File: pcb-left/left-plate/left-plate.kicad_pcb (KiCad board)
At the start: 2 copper layers, 197.4 x 119.6 mm, 71 parts, among them SW0 SW_PUSH, SW1 SW_PUSH, SW10 SW_PUSH, SW11 SW_PUSH, SW12 SW_PUSH, SW13 SW_PUSH, SW14 SW_PUSH, SW15 SW_PUSH, SW16 SW_PUSH, SW17 SW_PUSH, SW18 SW_PUSH, SW19 SW_PUSH, SW2 SW_PUSH, SW20 SW_PUSH, SW21 SW_PUSH, SW22 SW_PUSH, SW23 SW_PUSH, SW24 SW_PUSH, SW25 SW_PUSH, SW26 SW_PUSH, SW27 SW_PUSH, SW28 SW_PUSH, SW29 SW_PUSH, SW3 SW_PUSH, SW30 SW_PUSH, SW31 SW_PUSH, SW4 SW_PUSH, SW5 SW_PUSH, SW6 SW_PUSH, SW7 SW_PUSH, SW8 SW_PUSH, SW9 SW_PUSH

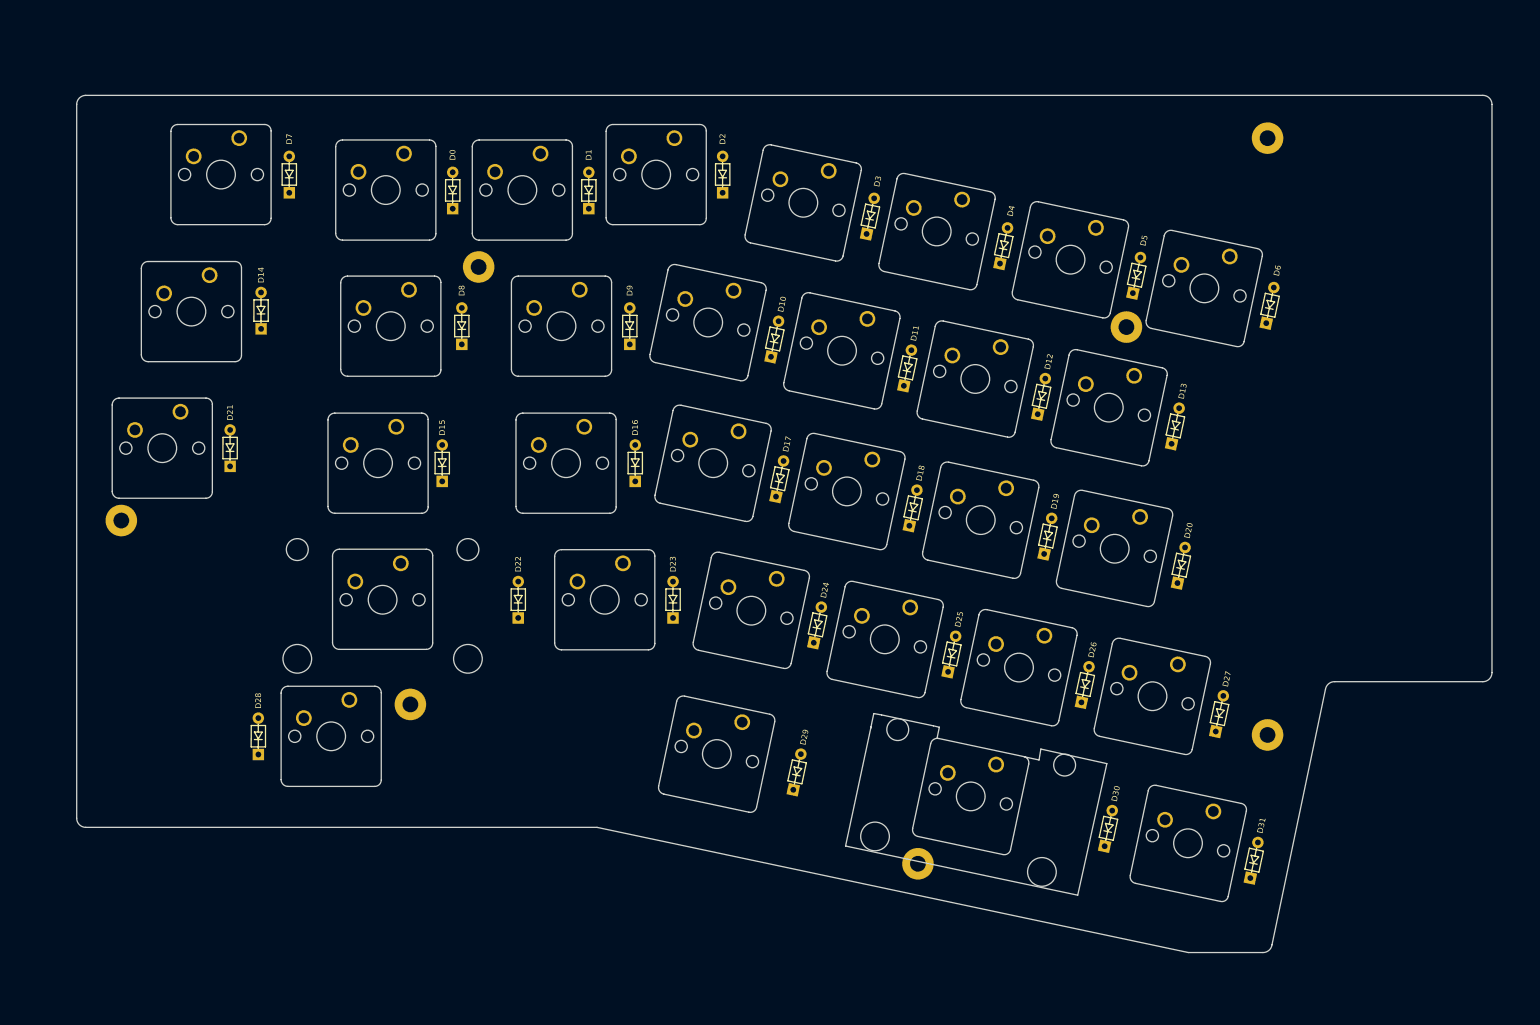
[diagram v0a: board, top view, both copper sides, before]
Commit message: update
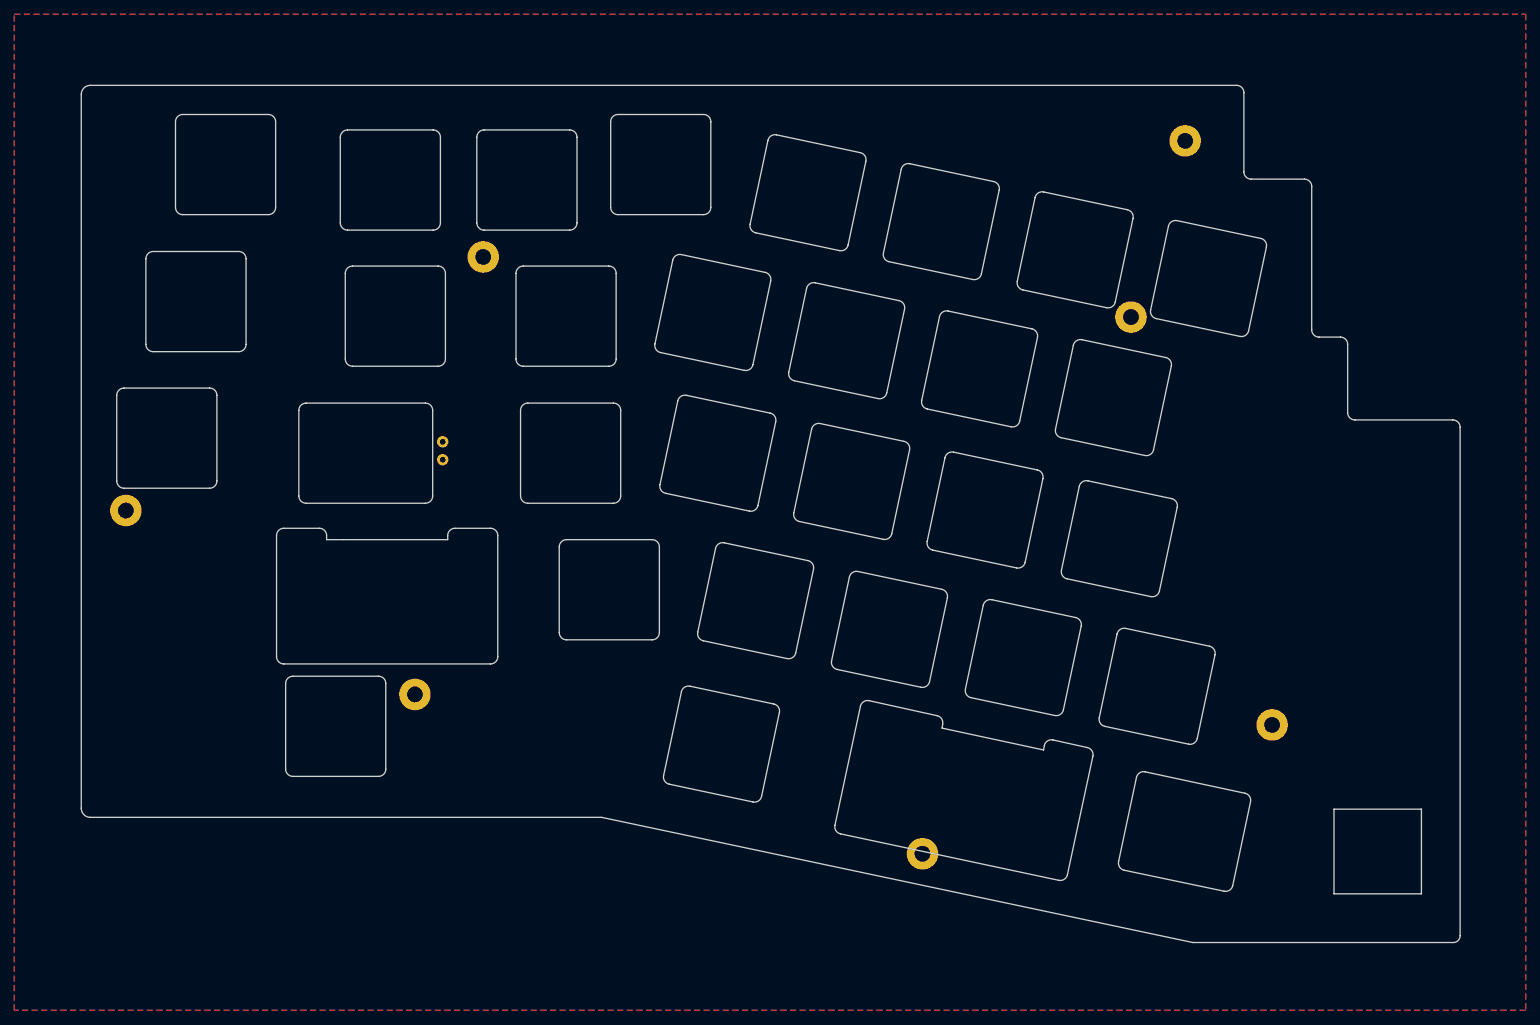
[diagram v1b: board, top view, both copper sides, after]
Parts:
- removed D0, D1, D10, D11, D12, D13, D14, D15, D16, D17, D18, D19, D2, D20, D21, D22, D23, D24, D25, D26, D27, D28, D29, D3, D30, D31, D4, D5, D6, D7, D8, D9: D, cftkb:D_DO-35_SOD27_P5.08mm_Horizontal
- removed SW0, SW1, SW10, SW11, SW12, SW13, SW14, SW16, SW17, SW18, SW19, SW2, SW20, SW21, SW23, SW24, SW25, SW26, SW27, SW3, SW31, SW4, SW5, SW6, SW7, SW9: SW_PUSH, cftkb:SW_Cherry_MX1A_1.00u_PCB-NOSCREEN
- removed SW15: SW_PUSH, cftkb:SW_Cherry_MX1A_1.75u_PCBNOSCREEN
- removed SW22, SW30: SW_PUSH, cftkb:SW_Cherry_MX1A_2.25u_PCBNOSCREEN
- removed SW28, SW29, SW8: SW_PUSH, cftkb:SW_Cherry_MX1A_1.50u_PCBNOSCREEN
- added C1: Device_C_Small, cftkb:C_Disc_D3.0mm_W1.6mm_P2.50mm, B.Cu at (99.5, 84.3)
- moved TH1 11.5 mm to (203.1, 42.3)
- moved TH6 1.53 mm to (195.5, 66.9)
- moved TH2 1.53 mm to (55.3, 93.9)
- moved TH4 1.53 mm to (95.6, 119.5)
- moved TH5 1.53 mm to (215.2, 123.8)
- moved TH7 1.53 mm to (166.4, 141.7)
- moved TH3 1.53 mm to (105.2, 58.5)
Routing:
- added copper zone on B.Cu, net GND
- added copper zone on F.Cu, net GND
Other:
- board size 197.4 x 119.6 mm -> 192.3 x 119.6 mm
